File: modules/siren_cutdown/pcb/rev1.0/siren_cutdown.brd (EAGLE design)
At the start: 30.1 x 32.5 mm, 20 parts, among them IC2 PICAXE-08M2

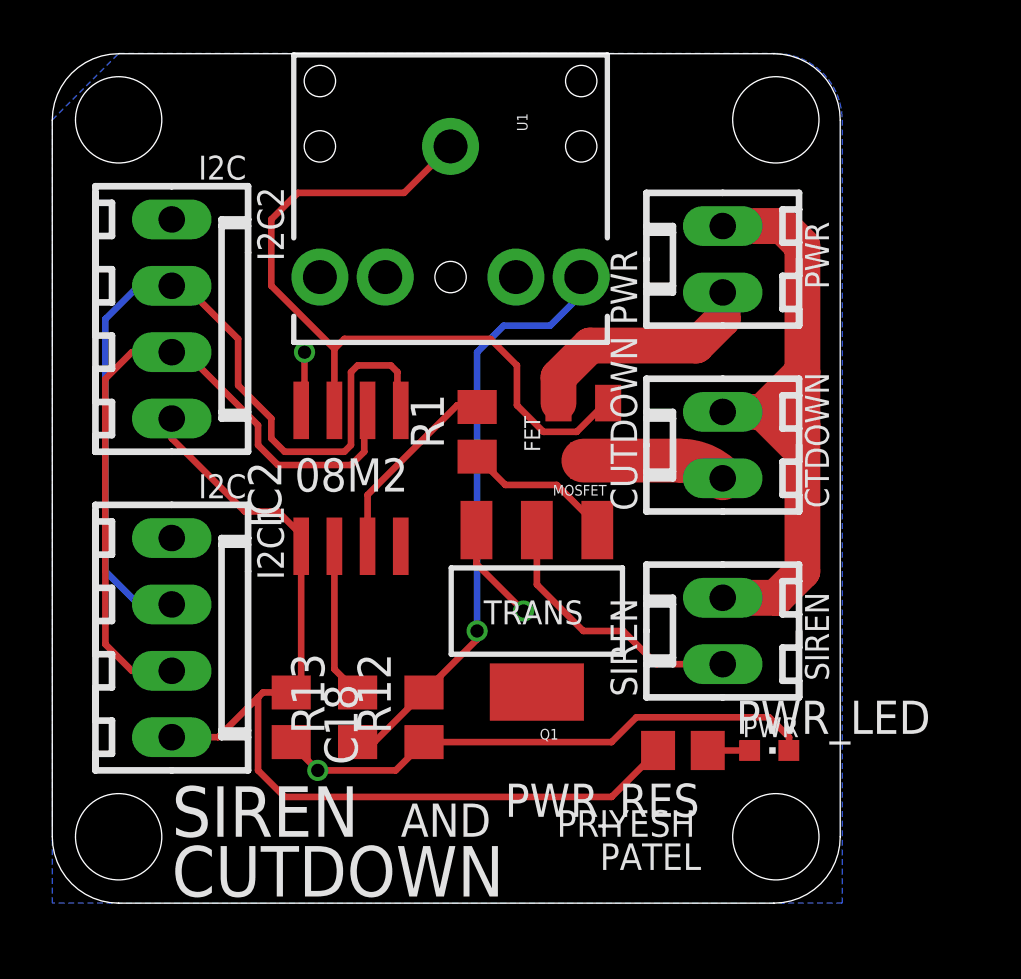
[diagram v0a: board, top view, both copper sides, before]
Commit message: siren pcb
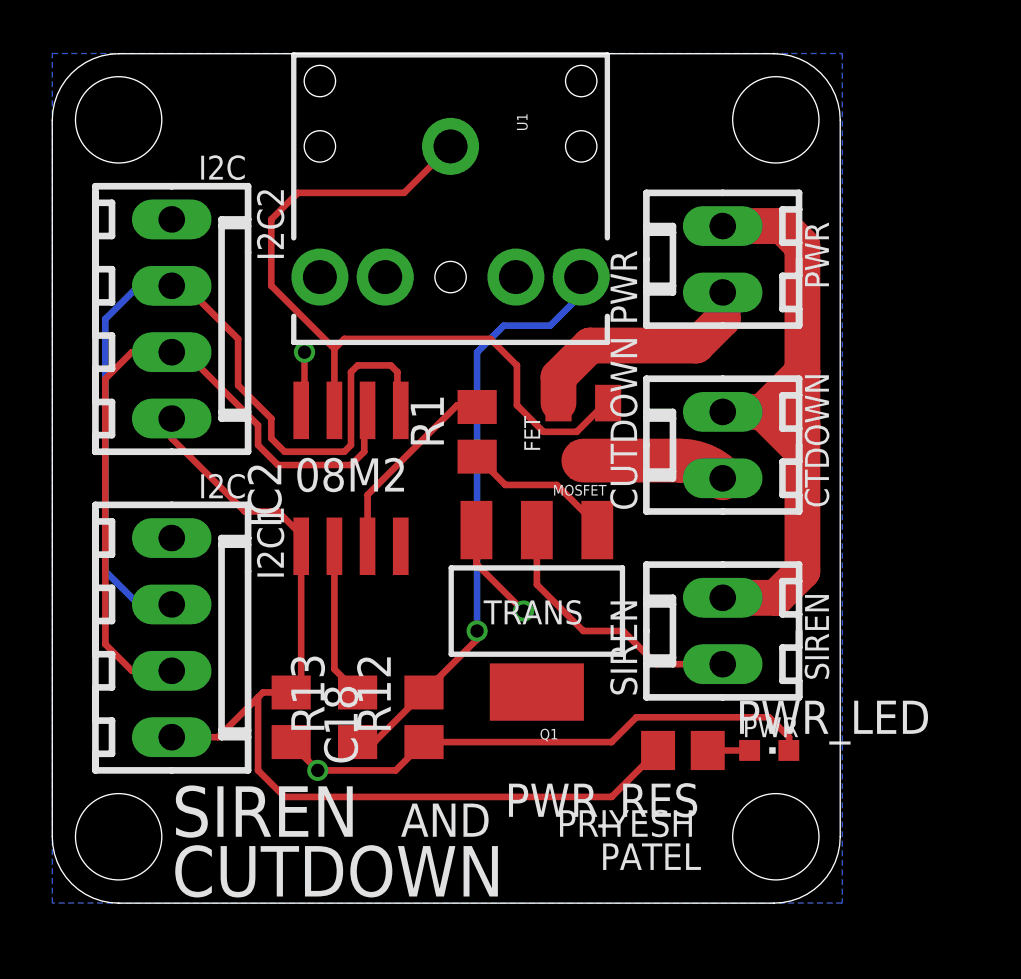
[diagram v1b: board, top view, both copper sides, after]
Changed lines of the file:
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@@
 <setting verticaltext="up"/>
 </settings>
-<grid distance="0.01" unitdist="inch" unit="inch" style="lines" multiple="1" display="yes" altdistance="0.005" altunitdist="inch" altunit="inch"/>
+<grid distance="0.05" unitdist="inch" unit="inch" style="lines" multiple="1" display="yes" altdistance="0.005" altunitdist="inch" altunit="inch"/>
 <layers>
 <layer number="1" name="Top" color="4" fill="1" visible="yes" active="yes"/>
@@
 <polygon width="0.254" layer="16" isolate="0.254">
 <vertex x="0" y="0"/>
-<vertex x="0" y="29.972"/>
-<vertex x="2.54" y="32.512"/>
-<vertex x="27.686" y="32.512" curve="-90"/>
-<vertex x="30.226" y="29.972"/>
+<vertex x="0" y="32.512"/>
+<vertex x="30.226" y="32.512"/>
 <vertex x="30.226" y="0"/>
 </polygon>
@@
 <wire x1="27.178" y1="18.796" x2="28.702" y2="20.32" width="1.3716" layer="1"/>
 <wire x1="27.178" y1="18.796" x2="28.702" y2="17.272" width="1.3716" layer="1"/>
-<wire x1="28.702" y1="17.272" x2="27.178" y2="18.796" width="0" layer="19" extent="1-16"/>
 </signal>
 <signal name="CUTDOWN">
